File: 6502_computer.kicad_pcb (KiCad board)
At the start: 4 copper layers, 100 x 100 mm, 0 parts

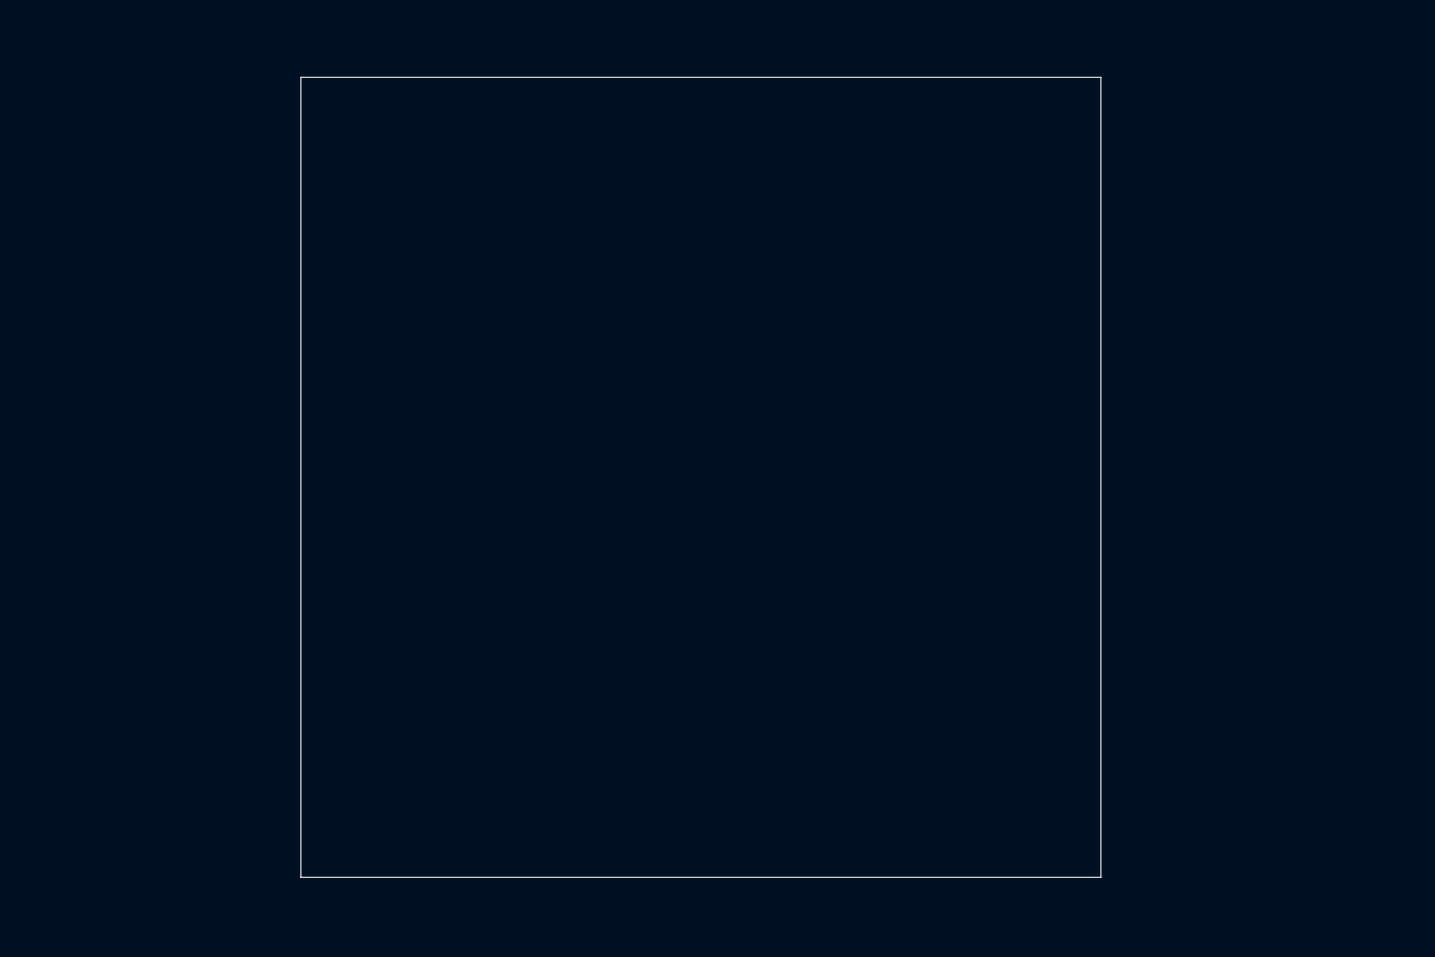
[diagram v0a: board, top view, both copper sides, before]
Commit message: First board
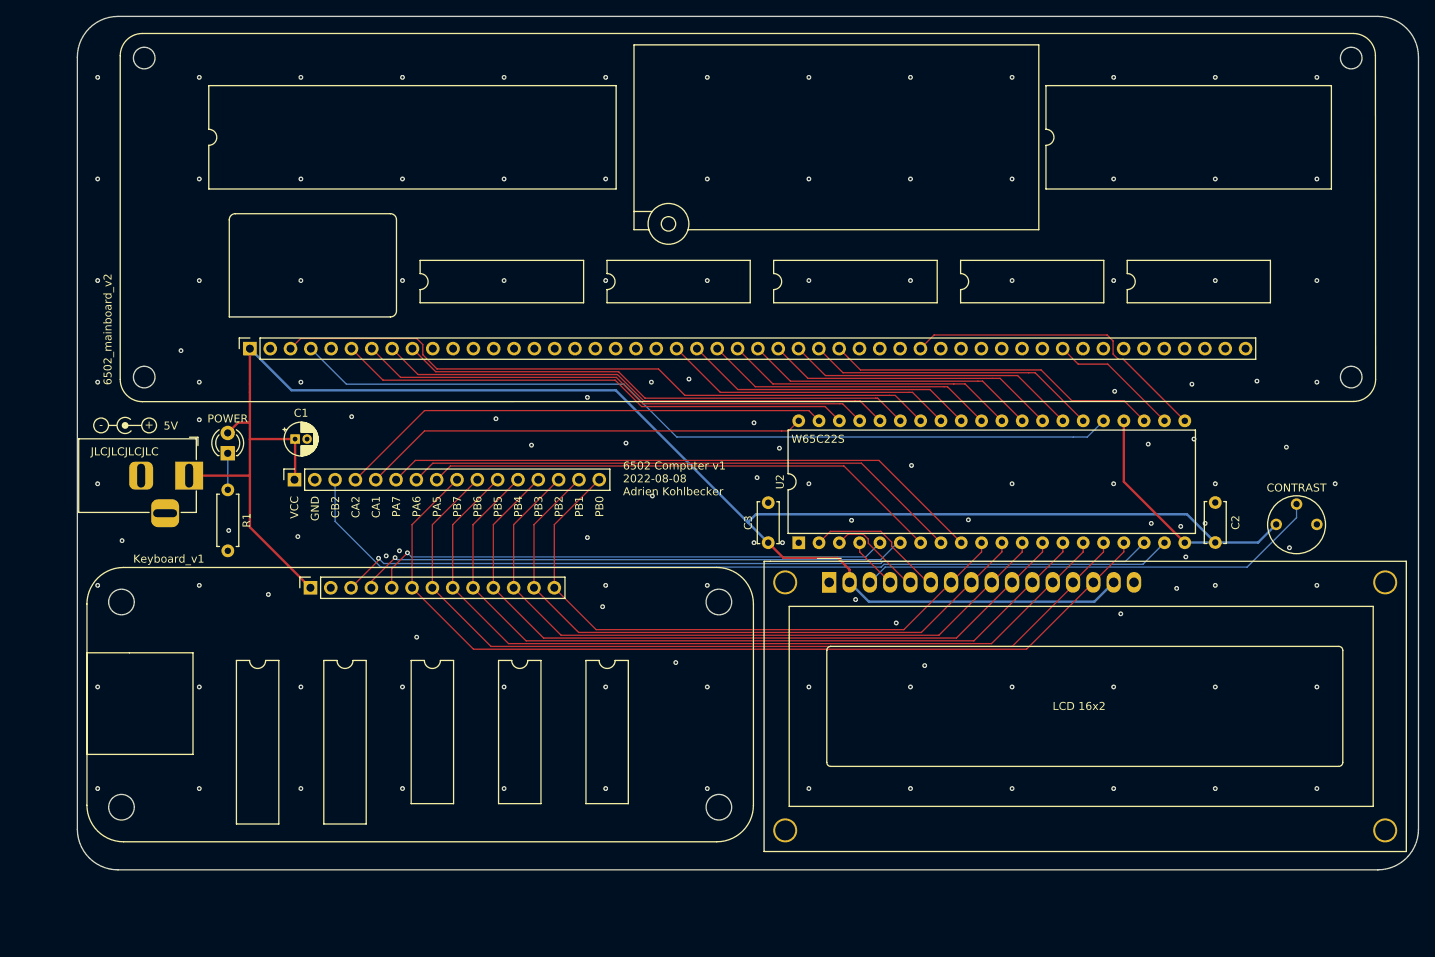
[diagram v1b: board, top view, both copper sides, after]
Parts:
- added C1: 10u, Capacitor_THT:CP_Radial_D4.0mm_P1.50mm, F.Cu at (100.9, 96.0)
- added C2: 100n, Capacitor_THT:C_Disc_D5.0mm_W2.5mm_P5.00mm, F.Cu at (215.9, 108.9)
- added C3: 100n, Capacitor_THT:C_Disc_D5.0mm_W2.5mm_P5.00mm, F.Cu at (160.0, 109.0)
- added D1: POWER, LED_THT:LED_D3.0mm, F.Cu at (92.5, 97.8)
- added DS1: WC1602A, Display:WC1602A, F.Cu at (167.6, 113.9)
- added J1: Barrel_Jack_Switch, Connector_BarrelJack:BarrelJack_Horizontal, F.Cu at (87.6, 100.6)
- added J2: Conn_01x16, Connector_PinSocket_2.54mm:PinSocket_1x16_P2.54mm_Vertical, F.Cu at (100.8, 101.1)
- added R1: 1k, Resistor_THT:R_Axial_DIN0207_L6.3mm_D2.5mm_P7.62mm_Horizontal, F.Cu at (92.5, 102.4)
- added REF**: Symbol_Barrel_Polarity, Symbol:Symbol_Barrel_Polarity, F.Cu at (79.6, 94.2)
- added RV1: 4.7k, Potentiometer_THT:Potentiometer_Vishay_T7-YA_Single_Vertical, F.Cu at (228.6, 106.7)
- added U1: 6502_mainboard_v2, AK's_Footprints:Mainboard v2, F.Cu at (162.8, 67.8)
- added U2: W65C22SxP, Package_DIP:DIP-40_W15.24mm, F.Cu at (163.8, 109.0)
- added U3: Keyboard_v1, AK's_Footprints:Keyboard v1, F.Cu at (118.1, 129.9)
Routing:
- net VCC: track 0.00 -> 268.8 mm
- net /PB7: track 0.00 -> 114.2 mm
- net /VIA_CB2: track 0.00 -> 112.5 mm
- net /PB6: track 0.00 -> 109.0 mm
- net /CLK: track 0.00 -> 104.5 mm
- net /PB5: track 0.00 -> 103.4 mm
- net /KB_IRQ: track 0.00 -> 102.2 mm, vias 0 -> 1
- net /PB4: track 0.00 -> 98.1 mm
- net /PB3: track 0.00 -> 92.7 mm
- net /PB2: track 0.00 -> 87.3 mm
- net /~{RST}: track 0.00 -> 84.3 mm
- net /PB1: track 0.00 -> 82.0 mm
- net /PB0: track 0.00 -> 76.6 mm
- net /VIA_PA7: track 0.00 -> 75.9 mm
- net /VIA_PA6: track 0.00 -> 70.5 mm
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- added copper zone on In1.Cu, net GND
- added copper zone on In2.Cu, net GND
- removed copper zone on In1.Cu, net (none)
- removed copper zone on In2.Cu, net (none)
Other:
- board size 100 x 100 mm -> 167.6 x 106.7 mm
- board text added: "+"
- board text added: "-"
- board text added: "5V"
- board text added: "6502 Computer v1 2022-08-08 Adrien Kohlbecker"
- board text added: "CA1"
- board text added: "CA2"
- board text added: "CB2"
- board text added: "CONTRAST"
- board text added: "GND"
- board text added: "JLCJLCJLCJLC"
- board text added: "LCD 16x2"
- board text added: "PA5"
- board text added: "PA6"
- board text added: "PA7"
- board text added: "PB0"
- board text added: "PB1"
- board text added: "PB2"
- board text added: "PB3"
- board text added: "PB4"
- board text added: "PB5"
- board text added: "PB6"
- board text added: "PB7"
- board text added: "VCC"
- board text added: "W65C22S"

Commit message: Update
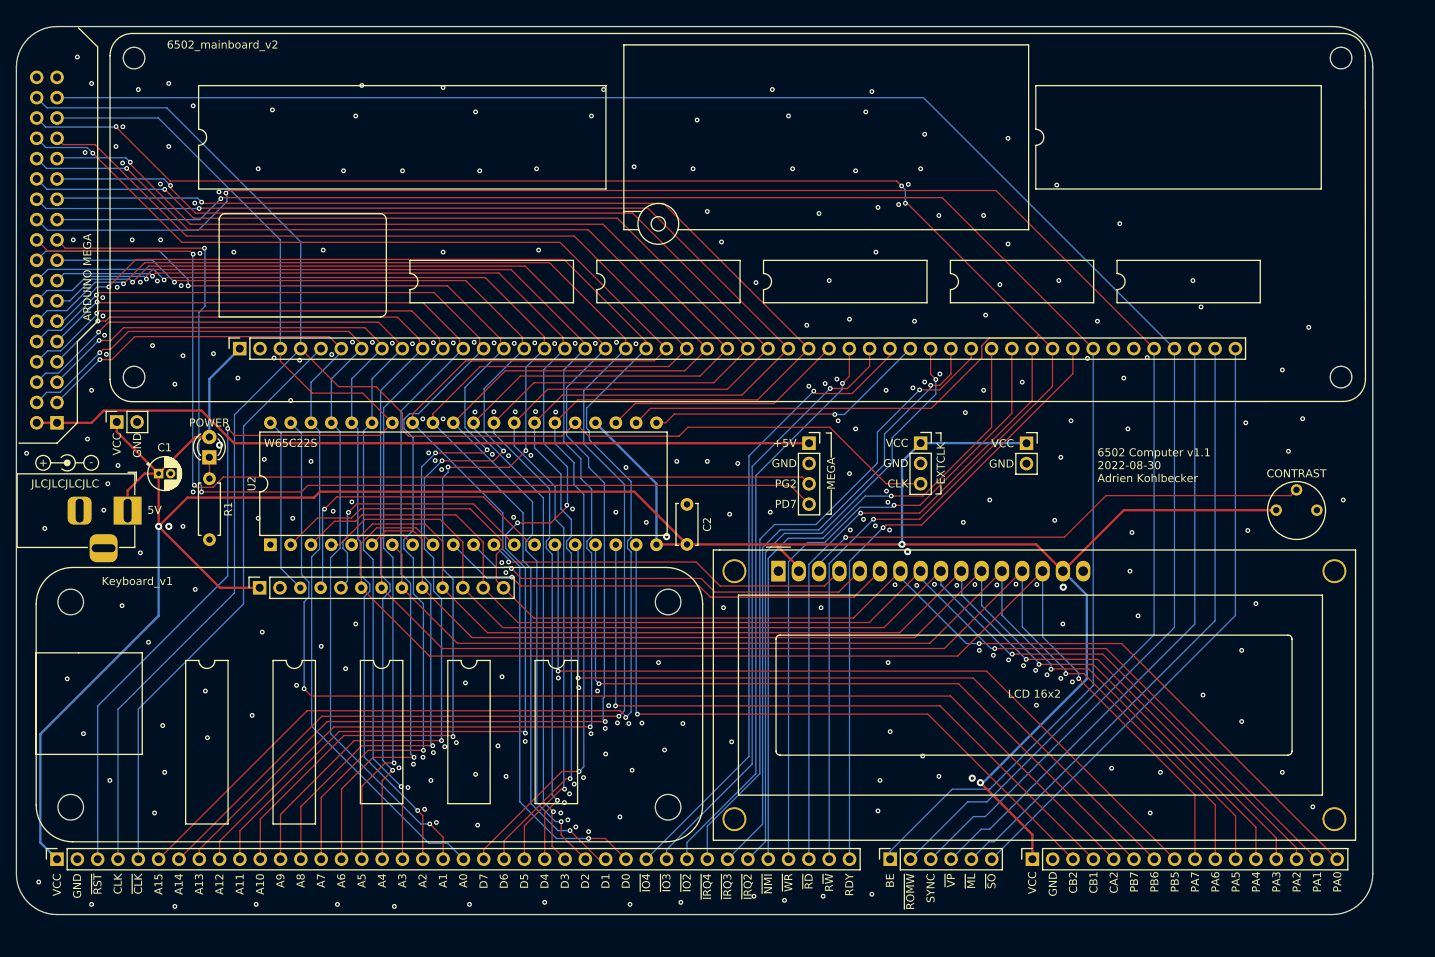
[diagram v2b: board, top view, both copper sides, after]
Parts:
- removed C3: 100n, Capacitor_THT:C_Disc_D5.0mm_W2.5mm_P5.00mm
- added J3: Mega, Connector_PinHeader_2.54mm:PinHeader_2x18_P2.54mm_Vertical, F.Cu at (71.1, 94.0)
- added J4: Mega, Connector_PinSocket_2.54mm:PinSocket_1x04_P2.54mm_Vertical, F.Cu at (165.1, 96.5)
- added J5: Clock, Connector_PinSocket_2.54mm:PinSocket_1x03_P2.54mm_Vertical, F.Cu at (179.1, 96.5)
- added J6: Conn_01x40, Connector_PinSocket_2.54mm:PinSocket_1x40_P2.54mm_Vertical, F.Cu at (71.1, 148.5)
- added J7: Conn_01x06, Connector_PinSocket_2.54mm:PinSocket_1x06_P2.54mm_Vertical, F.Cu at (175.3, 148.5)
- added J8: Conn_01x02, Connector_PinSocket_2.54mm:PinSocket_1x02_P2.54mm_Vertical, F.Cu at (78.6, 93.9)
- added J9: Conn_01x02, Connector_PinSocket_2.54mm:PinSocket_1x02_P2.54mm_Vertical, F.Cu at (192.3, 96.5)
- RV1: value 4.7k -> 10k
- moved J2 103.7 mm to (193.0, 148.5)
- moved U2 66.0 mm to (97.8, 109.2)
- moved C2 66.0 mm to (149.9, 109.2)
- moved C1 17.6 mm to (83.8, 100.3)
- moved J1 8.85 mm to (79.9, 105.0)
- moved REF** 8.70 mm to (72.4, 99.1), turned to 180 degrees
- moved DS1 6.50 mm to (161.3, 112.5)
- moved U3 6.35 mm to (111.8, 129.9)
- moved R1 2.69 mm to (90.2, 101.0)
- moved D1 2.35 mm to (90.2, 98.3)
- moved RV1 1.78 mm to (228.6, 104.9)
- moved U1 1.27 mm to (161.5, 67.8)
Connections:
- net /CS_VIA renamed /~{CS_VIA}
- net /IRQ_VIA renamed /~{IRQ_VIA}
- DS1 pad 10: /PB3 -> /PA3
- DS1 pad 11: /PB4 -> /PA4
- DS1 pad 12: /PB5 -> /PA5
- DS1 pad 13: /PB6 -> /PA6
- DS1 pad 14: /PB7 -> /PA7
- DS1 pad 7: /PB0 -> /PA0
- DS1 pad 8: /PB1 -> /PA1
- DS1 pad 9: /PB2 -> /PA2
- J2 pad 10: /PB6 -> /PA6
- J2 pad 11: /PB5 -> /PA5
- J2 pad 12: /PB4 -> /PA4
- J2 pad 13: /PB3 -> /PA3
- J2 pad 14: /PB2 -> /PA2
- J2 pad 15: /PB1 -> /PA1
- J2 pad 16: /PB0 -> /PA0
- J2 pad 4: /VIA_CA2 -> /VIA_CB1
- J2 pad 5: /VIA_CA1 -> /VIA_CA2
- J2 pad 6: /VIA_PA7 -> /VIA_PB7
- J2 pad 7: /VIA_PA6 -> /VIA_PB6
- J2 pad 8: /VIA_PA5 -> /VIA_PB5
- J2 pad 9: /PB7 -> /PA7
- U1 pad 10: unconnected-(U1-Pad10) -> /A4
- U1 pad 11: unconnected-(U1-Pad11) -> /A5
- U1 pad 12: unconnected-(U1-Pad12) -> /A6
- U1 pad 13: unconnected-(U1-Pad13) -> /A7
- U1 pad 14: unconnected-(U1-Pad14) -> /A8
- U1 pad 15: unconnected-(U1-Pad15) -> /A9
- U1 pad 16: unconnected-(U1-Pad16) -> /A10
- U1 pad 17: unconnected-(U1-Pad17) -> /A11
- U1 pad 18: unconnected-(U1-Pad18) -> /A12
- U1 pad 19: unconnected-(U1-Pad19) -> /A13
- U1 pad 20: unconnected-(U1-Pad20) -> /A14
- U1 pad 21: unconnected-(U1-Pad21) -> /A15
- U1 pad 31: unconnected-(U1-Pad31) -> /~{IO2}
- U1 pad 32: unconnected-(U1-Pad32) -> /~{IO3}
- U1 pad 33: unconnected-(U1-Pad33) -> /~{IO4}
- U1 pad 35: unconnected-(U1-Pad35) -> /~{IRQ2}
- U1 pad 36: unconnected-(U1-Pad36) -> /~{IRQ3}
- U1 pad 37: unconnected-(U1-Pad37) -> /~{IRQ4}
- U1 pad 38: unconnected-(U1-Pad38) -> /~{NMI}
- U1 pad 39: unconnected-(U1-Pad39) -> /~{WR}
- U1 pad 40: unconnected-(U1-Pad40) -> /~{RD}
- U1 pad 42: unconnected-(U1-Pad42) -> /RDY
- U1 pad 43: unconnected-(U1-Pad43) -> /BE
- U1 pad 46: unconnected-(U1-Pad46) -> /~{ROMW}
- U1 pad 47: unconnected-(U1-Pad47) -> /SYNC
- U1 pad 48: unconnected-(U1-Pad48) -> /~{VP}
- U1 pad 49: unconnected-(U1-Pad49) -> /~{ML}
- U1 pad 5: unconnected-(U1-Pad5) -> /~{CLK}
- U1 pad 50: unconnected-(U1-Pad50) -> /~{SO}
- U2 pad 10: /PB0 -> /LCD_E
- U2 pad 11: /PB1 -> /LCD_RW
- U2 pad 12: /PB2 -> /LCD_RS
- U2 pad 13: /PB3 -> /KB_E
- U2 pad 14: /PB4 -> /KB_VALID
- U2 pad 15: /PB5 -> /VIA_PB5
- U2 pad 16: /PB6 -> /VIA_PB6
- U2 pad 17: /PB7 -> /VIA_PB7
- U2 pad 18: /KB_IRQ -> /VIA_CB1
- U2 pad 2: /LCD_E -> /PA0
- U2 pad 3: /LCD_RW -> /PA1
- U2 pad 4: /LCD_RS -> /PA2
- U2 pad 40: /VIA_CA1 -> /KB_IRQ
- U2 pad 5: /KB_E -> /PA3
- U2 pad 6: /KB_VALID -> /PA4
- U2 pad 7: /VIA_PA5 -> /PA5
- U2 pad 8: /VIA_PA6 -> /PA6
- U2 pad 9: /VIA_PA7 -> /PA7
- U3 pad 10: /PB3 -> /PA3
- U3 pad 11: /PB2 -> /PA2
- U3 pad 12: /PB1 -> /PA1
- U3 pad 13: /PB0 -> /PA0
- U3 pad 6: /PB7 -> /PA7
- U3 pad 7: /PB6 -> /PA6
- U3 pad 8: /PB5 -> /PA5
- U3 pad 9: /PB4 -> /PA4
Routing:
- net /R~{W}: track 16.5 -> 274.5 mm, vias 0 -> 4
- net /SYNC: track 0.00 -> 230.0 mm
- net /~{ROMW}: track 0.00 -> 229.1 mm, vias 0 -> 1
- net /BE: track 0.00 -> 215.5 mm, vias 0 -> 1
- net /A15: track 0.00 -> 200.7 mm, vias 0 -> 2
- net /A14: track 0.00 -> 194.9 mm, vias 0 -> 2
- net /A13: track 0.00 -> 184.4 mm, vias 0 -> 2
- net /A12: track 0.00 -> 180.0 mm, vias 0 -> 2
- net /A11: track 0.00 -> 170.3 mm, vias 0 -> 4
- net /D7: track 36.8 -> 199.9 mm, vias 0 -> 2
- net /A10: track 0.00 -> 161.6 mm, vias 0 -> 4
- net /D6: track 36.8 -> 198.0 mm, vias 0 -> 2
- net /PA0: track 0.00 -> 160.1 mm, vias 0 -> 1
- net /D0: track 36.8 -> 195.0 mm, vias 0 -> 2
- net /D5: track 36.8 -> 192.9 mm, vias 0 -> 2
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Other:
- board size 167.6 x 106.7 mm -> 169.5 x 111 mm
- board text added: "+5V"
- board text added: "6502 Computer v1.1 2022-08-30 Adrien Kohlbecker"
- board text added: "= PA0..7 = PC0..7 = PL0..7 = PB0 = PB1 = PB2 = PB3 = PG0 = PG1"
- board text added: "A0"
- board text added: "A1"
- board text added: "A10"
- board text added: "A11"
- board text added: "A12"
- board text added: "A13"
- board text added: "A14"
- board text added: "A15"
- board text added: "A2"
- board text added: "A3"
- board text added: "A4"
- board text added: "A5"
- board text added: "A6"
- board text added: "A7"
- board text added: "A8"
- board text added: "A9"
- board text added: "ARDUINO MEGA"
- board text added: "BE"
- board text added: "CB1"
- board text added: "CLK"
- board text added: "D0"
- board text added: "D1"
- board text added: "D2"
- board text added: "D3"
- board text added: "D4"
- board text added: "D5"
- board text added: "D6"
- board text added: "D7"
- board text added: "EXTCLK"
- board text added: "MEGA"
- board text added: "Mega pin mapping ------------ A0..7 A8..15 D0..7 CLK SYNC R/W /RST /ROMW BE"
- board text added: "PA0"
- board text added: "PA1"
- board text added: "PA2"
- board text added: "PA3"
- board text added: "PA4"
- board text added: "PD7"
- board text added: "PG2"
- board text added: "RDY"
- board text added: "R~{W}"
- board text added: "SYNC"
- board text added: "~{CLK}"
- board text added: "~{IO2}"
- board text added: "~{IO3}"
- board text added: "~{IO4}"
- board text added: "~{IRQ2}"
- board text added: "~{IRQ3}"
- board text added: "~{IRQ4}"
- board text added: "~{ML}"
- board text added: "~{NMI}"
- board text added: "~{RD}"
- board text added: "~{ROMW}"
- board text added: "~{RST}"
- board text added: "~{SO}"
- board text added: "~{VP}"
- board text added: "~{WR}"
- board text removed: "6502 Computer v1 2022-08-08 Adrien Kohlbecker"
- board text removed: "CA1"
- board text removed: "PB0"
- board text removed: "PB1"
- board text removed: "PB2"
- board text removed: "PB3"
- board text removed: "PB4"
